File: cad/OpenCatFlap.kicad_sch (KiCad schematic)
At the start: 25 parts, among them P1 IR Outside, P2 Flap IR Outside, P3 Flap IR Inside, P4 Servo Outside, P5 Servo Inside, P6 RFID Inside, P7 RFID Outside, P8 PIR Outside, U1 TCRT5000L, U3 5V

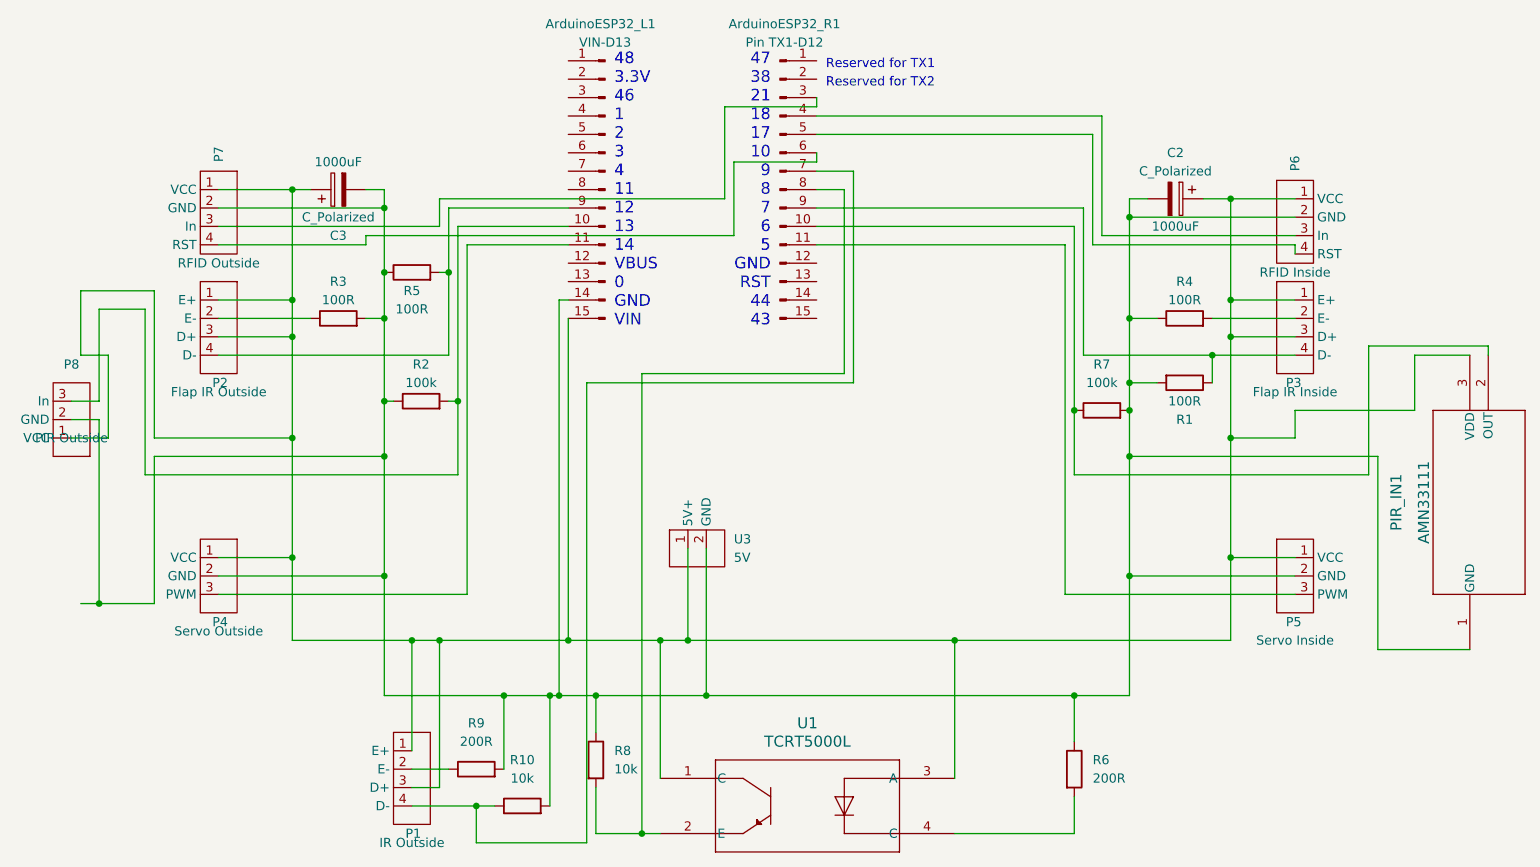
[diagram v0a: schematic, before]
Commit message: update schematics
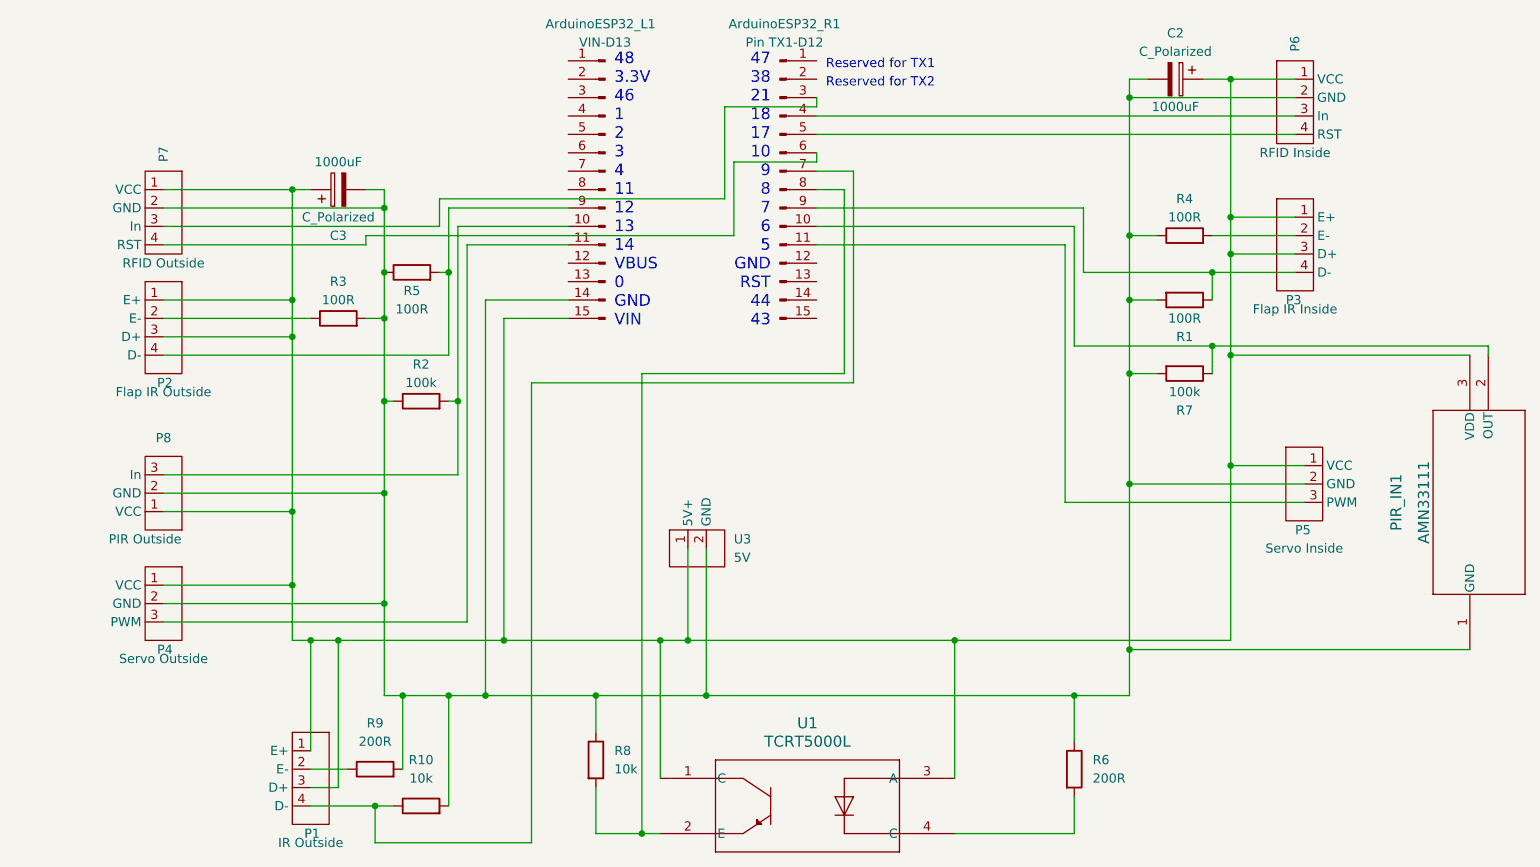
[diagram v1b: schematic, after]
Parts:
- P8: Comment on the part (none) -> Currently using AMN31112. AMN41122 might be a better fit?
- PIR_IN1: Commen on part (none) -> Currently using AMN31112. AMN41122 might be a better fit?
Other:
- moved on the sheet: C2, P1, P2, P3, P4, P5, P6, P7, P8, R1, R10, R4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
